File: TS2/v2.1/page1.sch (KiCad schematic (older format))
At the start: 16 parts, among them SW1 RESET, U1 555, U2 8 MHz, U3 74LS00, U4 74LS06, U5 74LS04, U6 68000

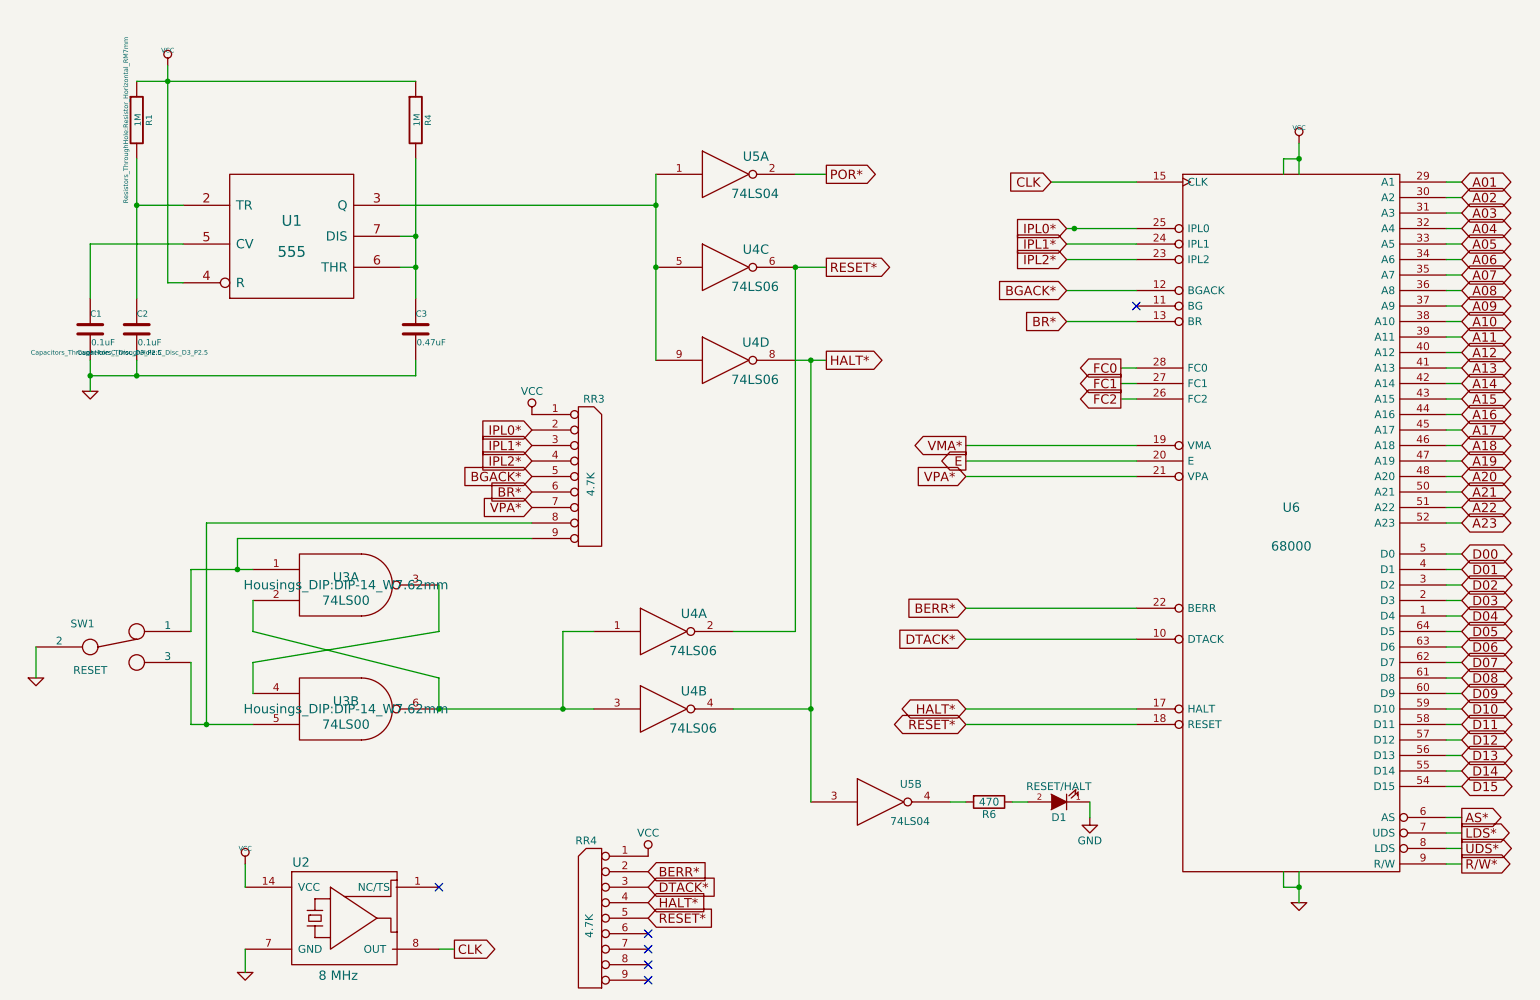
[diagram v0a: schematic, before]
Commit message: Rev 2.1.1 changes.
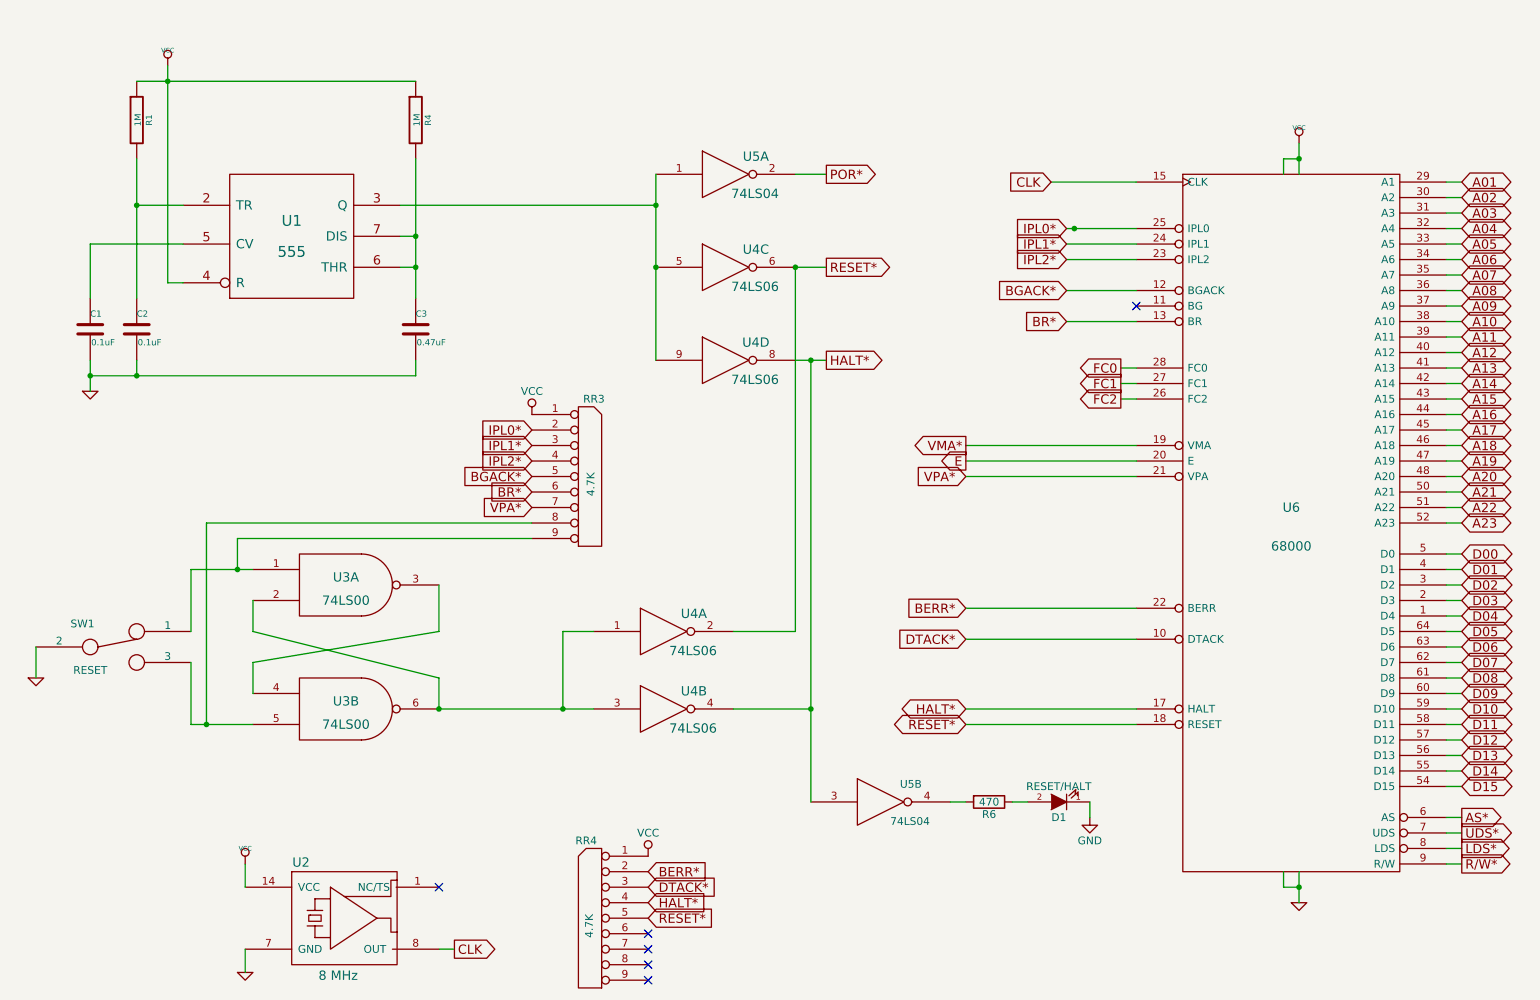
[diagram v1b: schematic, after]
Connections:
- net LDS*: now also U6.8 (LDS); no longer U6.7 (UDS)
- net UDS*: now also U6.7 (UDS); no longer U6.8 (LDS)
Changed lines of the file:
@@
 Sheet 2 9
 Title "TS2 68000 Single Board Computer"
-Date "2017-02-17"
-Rev "2.1"
+Date "2017-05-29"
+Rev "2.1.1"
 Comp "Jeff Tranter"
 Comment1 "Reset, Halt, and Clock Control Circuits"
@@
 F 0 "U3" H 2800 4150 60  0000 C CNN
 F 1 "74LS00" H 2800 4000 60  0000 C CNN
-F 2 "Housings_DIP:DIP-14_W7.62mm" H 2800 4100 60  0000 C CNN
+F 2 "Housings_DIP:DIP-14_W7.62mm" V 2800 4100 60  0001 C CNN
 F 3 "~" H 2800 4100 60  0000 C CNN
 	1    2800 4100
@@
 F 0 "U3" H 2800 4950 60  0000 C CNN
 F 1 "74LS00" H 2800 4800 60  0000 C CNN
-F 2 "Housings_DIP:DIP-14_W7.62mm" H 2800 4900 60  0000 C CNN
+F 2 "Housings_DIP:DIP-14_W7.62mm" H 2800 4900 60  0001 C CNN
 F 3 "~" H 2800 4900 60  0000 C CNN
 	2    2800 4900
@@
 F 0 "R1" V 1530 1100 40  0000 C CNN
 F 1 "1M" V 1457 1101 40  0000 C CNN
-F 2 "Resistors_ThroughHole:Resistor_Horizontal_RM7mm" V 1380 1100 30  0000 C CNN
+F 2 "Resistors_ThroughHole:Resistor_Horizontal_RM7mm" V 1380 1100 30  0001 C CNN
 F 3 "~" H 1450 1100 30  0000 C CNN
 	1    1450 1100
@@
 F 0 "C1" H 1150 2550 40  0000 L CNN
 F 1 "0.1uF" H 1156 2365 40  0000 L CNN
-F 2 "Capacitors_ThroughHole:C_Disc_D3_P2.5" H 1188 2300 30  0000 C CNN
+F 2 "Capacitors_ThroughHole:C_Disc_D3_P2.5" H 1500 1700 30  0001 C CNN
 F 3 "~" H 1150 2450 60  0000 C CNN
 	1    1150 2450
@@
 F 0 "C2" H 1450 2550 40  0000 L CNN
 F 1 "0.1uF" H 1456 2365 40  0000 L CNN
-F 2 "Capacitors_ThroughHole:C_Disc_D3_P2.5" H 1488 2300 30  0000 C CNN
+F 2 "Capacitors_ThroughHole:C_Disc_D3_P2.5" H 1488 2300 30  0001 C CNN
 F 3 "~" H 1450 2450 60  0000 C CNN
 	1    1450 2450
@@
 A01
 Text GLabel 10000 5800 2    60   Output ~ 0
+LDS*
+Text GLabel 10000 5700 2    60   Output ~ 0
 UDS*
-Text GLabel 10000 5700 2    60   Output ~ 0
-LDS*
 Text GLabel 10000 5900 2    60   Output ~ 0
 R/W*
